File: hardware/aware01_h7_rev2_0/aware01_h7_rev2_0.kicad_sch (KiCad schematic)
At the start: 45 parts, among them J1 Conn_02x07_Odd_Even, J2 Conn_02x05_Odd_Even, SW3 PTS815, U1 LMR50410Y5FQDBVRQ1, U2 LM1117MP-3.3, U4 STM32H7A3RITx, U5 LM4040DIM3X-10, Y1 WE-XTAL 24.0MHz 50ppm

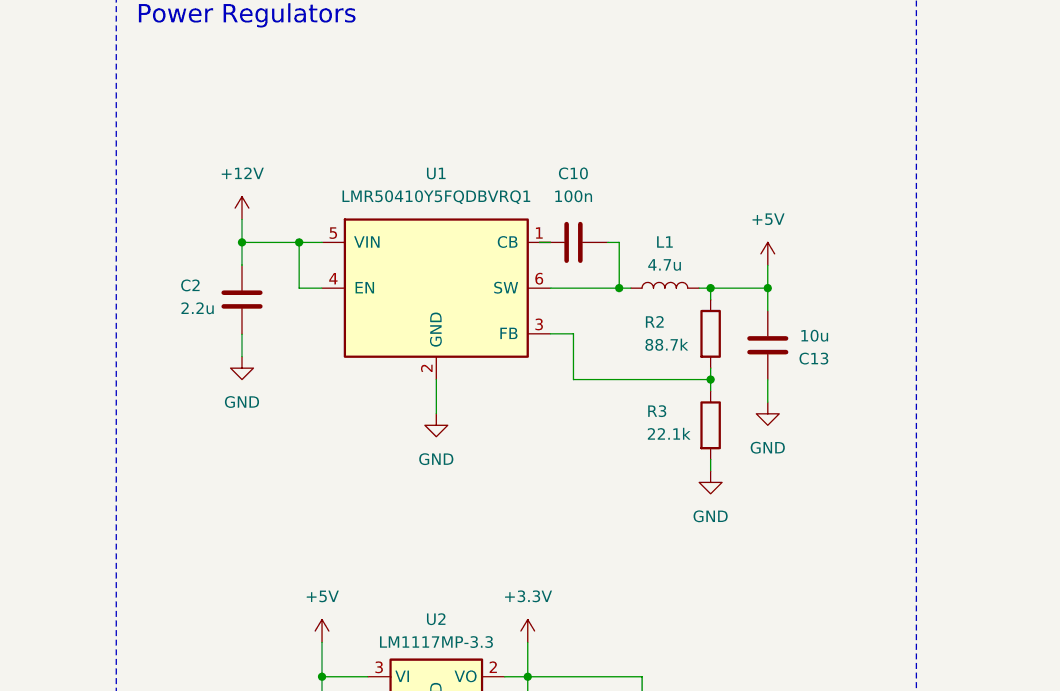
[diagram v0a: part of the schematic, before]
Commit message: hw: update BOM and layout
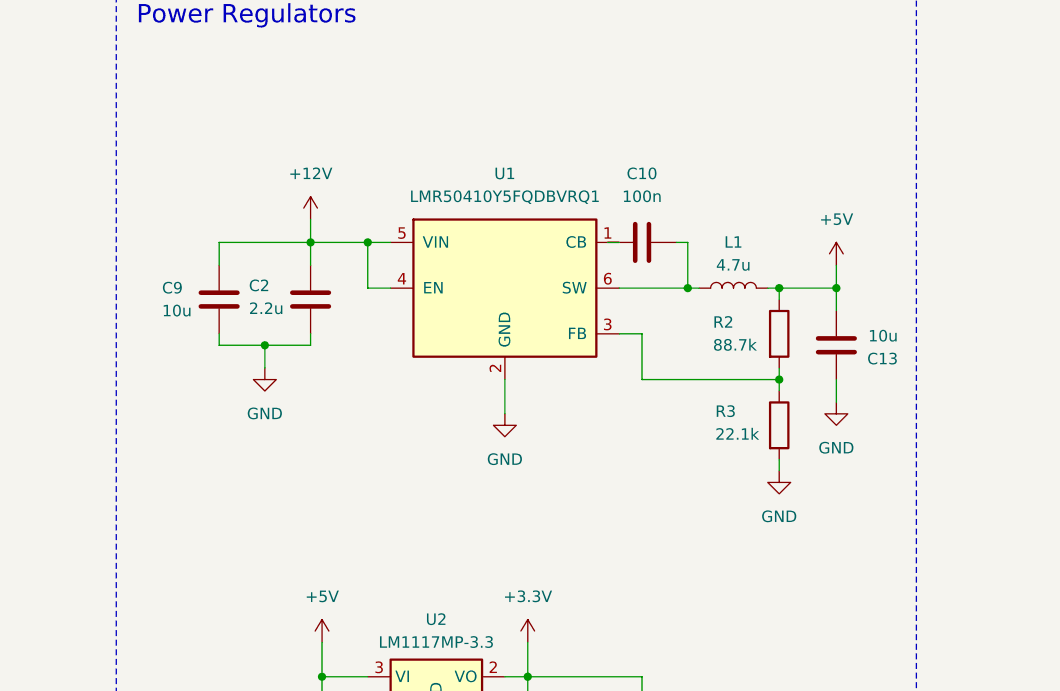
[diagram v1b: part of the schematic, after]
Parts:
- added C9: 10u, Capacitor_SMD:C_0603_1608Metric, symbol Device:C
- C13, C4, C8: Manufacturer_Part_Number GRM188R61E106KA73D -> GRM188R61E106KA73D
- C17: Manufacturer_Name KYOCERA AVX -> KYOCERA AVX; Manufacturer_Part_Number 04023U140GAT2A -> 04023U140GAT2A; Mouser Part Number 581-04023U140GAT2A -> 581-04023U140GAT2A
- C18, C22: Manufacturer_Name Walsin -> KYOCERA AVX; Manufacturer_Part_Number 0603B105M160CT -> KGM15AV51A105ZM; Mouser Part Number 791-0603B105M160CT -> 581-KGM15AV51A105ZM
- L1: Manufacturer_Part_Number SRR5228A-470M -> SRR5228A-4R7Y; Mouser Part Number 6521-SRR5228A-470M -> 6521-SRR5228A-4R7Y
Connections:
- net +12V: now also C9.1
- net GND: now also C9.2
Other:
- moved on the sheet: C10, C13, C2, L1, R2, R3, U1
